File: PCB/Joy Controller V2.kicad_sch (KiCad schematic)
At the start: 36 parts, among them J1 Conn_02x16_Odd_Even, J4 USB_C_Receptacle_USB2.0_16P, SW1 SW_Push, SW10 SW_Push, SW11 SW_Push, SW12 SW_Push, SW13 SW_Push, SW2 SW_Push, SW3 SW_Push, SW4 SW_Push, SW5 SW_Push, SW6 SW_Push, SW7 SW_Push, SW8 SW_Push, SW9 SW_Push, U1 COM-09032, U2 COM-09032

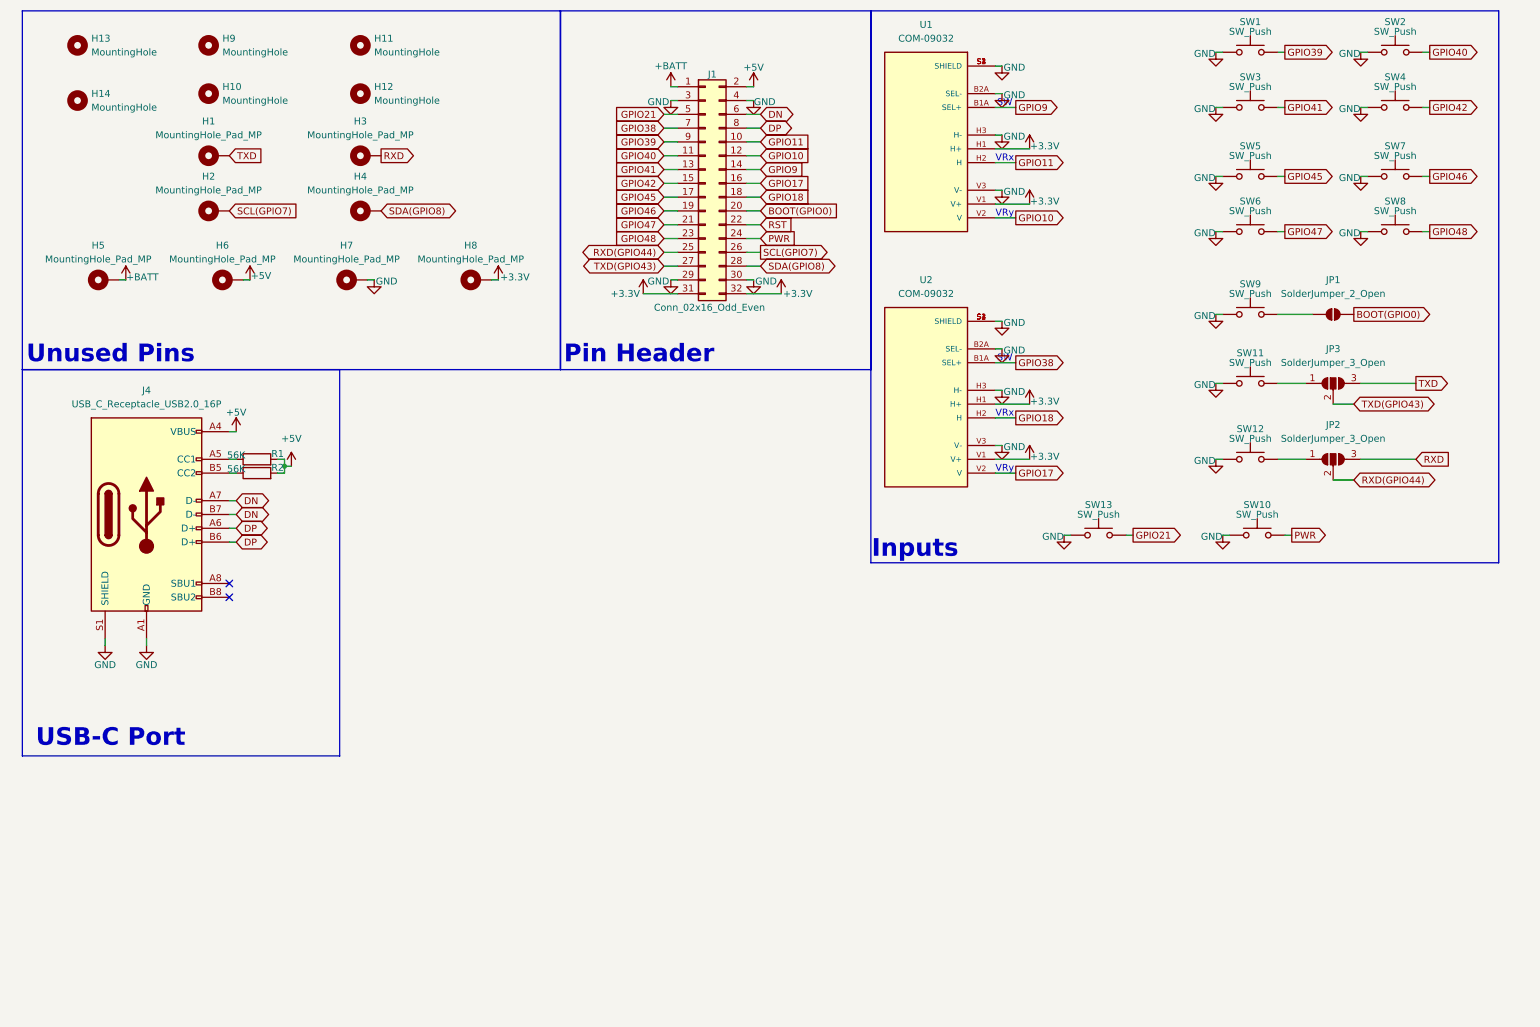
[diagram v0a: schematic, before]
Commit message: Add files via upload
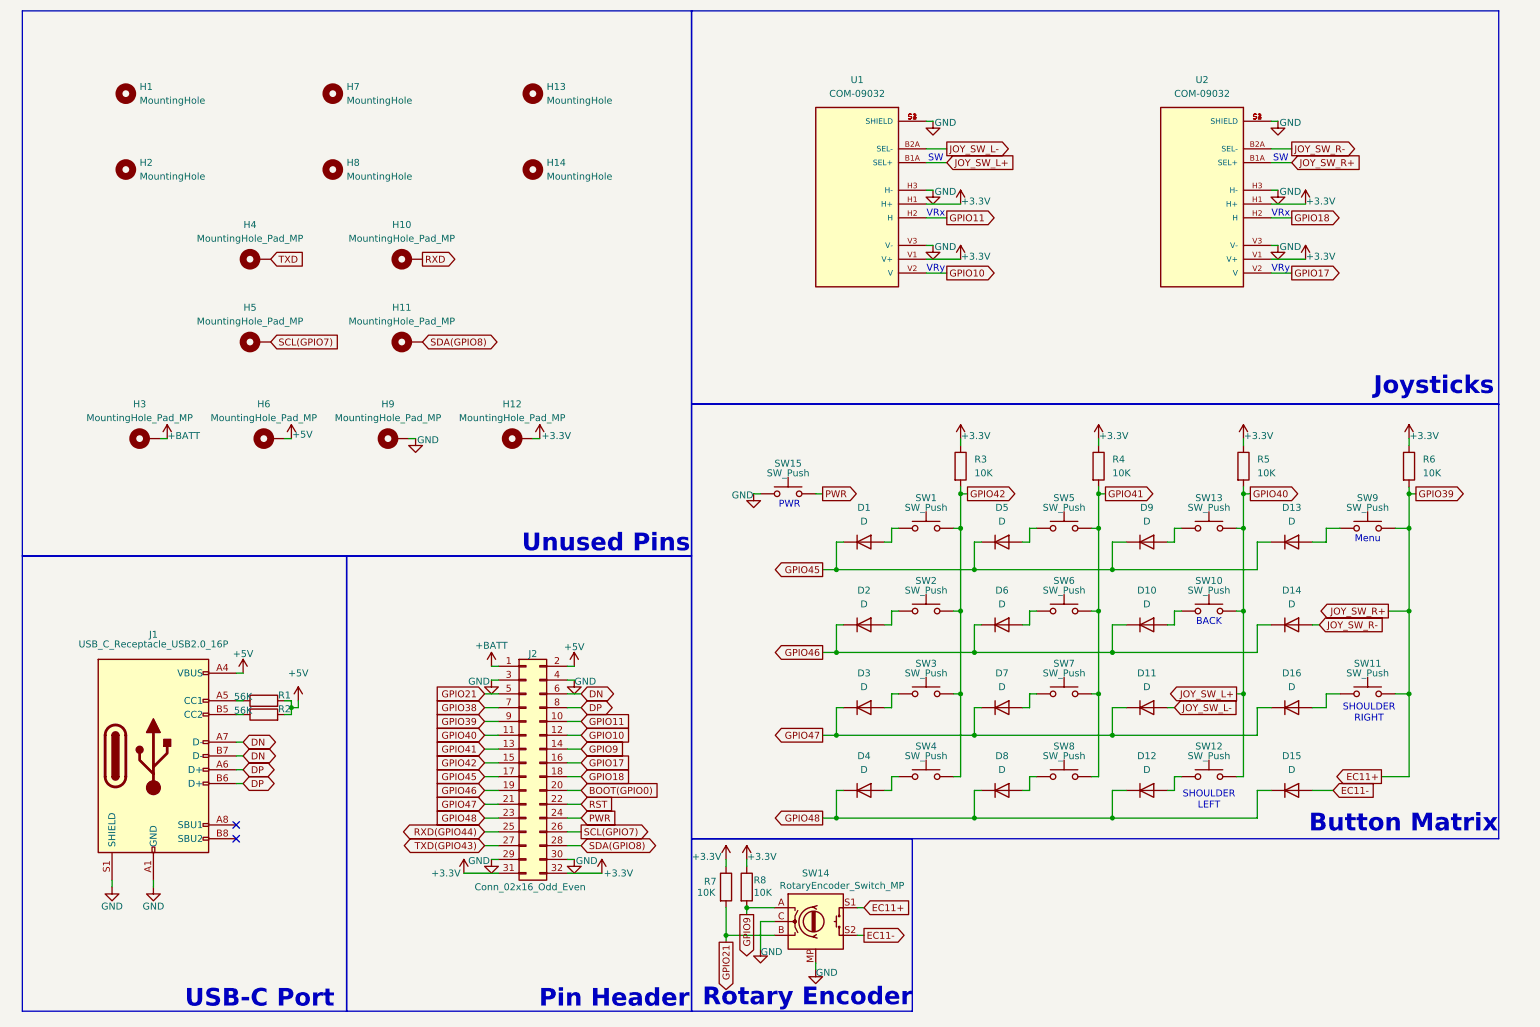
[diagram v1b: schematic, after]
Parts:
- removed JP1: SolderJumper_2_Open, Jumper:SolderJumper-2_P1.3mm_Open_RoundedPad1.0x1.5mm, symbol Jumper:SolderJumper_2_Open
- removed JP2, JP3: SolderJumper_3_Open, Jumper:SolderJumper-3_P1.3mm_Open_RoundedPad1.0x1.5mm, symbol Jumper:SolderJumper_3_Open
- added D1, D10, D11, D12, D13, D14, D15, D16, D2, D3, D4, D5, D6, D7, D8, D9: D, Diode_SMD:D_SOD-323, symbol Device:D
- added R3, R4, R5, R6, R7, R8: 10K, Resistor_SMD:R_0603_1608Metric, symbol Device:R
- added SW13: SW_Push, Button_Switch_THT:SW_Tactile_SKHH_Angled, symbol Switch:SW_Push
- added SW14: RotaryEncoder_Switch_MP, Rotary_Encoder:RotaryEncoder_Alps_EC11E-Switch_Vertical_H20mm, symbol Device:RotaryEncoder_Switch_MP
- renumbered H13 to H1, H3 to H10, H4 to H11, H8 to H12, H11 to H13, H12 to H14, H14 to H2, H5 to H3, H1 to H4, H2 to H5, H9 to H7, H10 to H8, H7 to H9, J4 to J1, J1 to J2, SW9 to SW10, SW10 to SW15, SW3 to SW2, SW5 to SW3, SW7 to SW4, SW2 to SW5, SW4 to SW6, SW6 to SW7, SW13 to SW9
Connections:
- net +3.3V: now also R3.1, R4.1, R5.1, R6.1, R7.1, R8.1
- net GND: now also SW14.C, SW14.MP; no longer SW1.1, SW10.1, SW11.1, SW12.1, SW2.1, SW3.1, SW4.1, SW5.1, SW6.1, SW7.1, SW8.1, SW9.1, U1.B2A (SEL-), U2.B2A (SEL-)
- net GPIO21: now also R7.2, SW14.B; no longer SW9.2
- net GPIO38: no longer U2.B1A (SEL+)
- net GPIO40: now also SW10.2, SW12.2, U1.B1A (SEL+), R5.2, SW13.2; no longer SW5.2
- net GPIO41: now also SW5.2, SW6.2, SW7.2, SW8.2, R4.2; no longer SW2.2
- net GPIO42: now also SW1.2, SW2.2, SW3.2, SW4.2, R3.2; no longer SW6.2
- net GPIO45: now also D1.1 (K), D13.1 (K), D5.1 (K), D9.1 (K); no longer SW3.2
- net GPIO46: now also D10.1 (K), D14.1 (K), D2.1 (K), D6.1 (K); no longer SW4.2
- net GPIO47: now also D11.1 (K), D16.1 (K), D3.1 (K), D7.1 (K); no longer SW7.2
- net GPIO48: now also D12.1 (K), D15.1 (K), D4.1 (K), D8.1 (K); no longer SW8.2
- net GPIO9: now also R8.2, SW14.A; no longer U1.B1A (SEL+)
- net EC11+: now reaches SW11.2
- net EC11+: now also J2.9 (Pin_9), SW9.2, U2.B1A (SEL+), R6.2, SW14.S1
- removed net GPIO39: J2.9 (Pin_9), SW1.2
- new net: D13.2 (A), SW9.1
- new net: D16.2 (A), SW11.1
- new net: D9.2 (A), SW13.1
- new net: D4.2 (A), SW4.1
- new net: D7.2 (A), SW7.1
- new net: D1.2 (A), SW1.1
- new net: D6.2 (A), SW6.1
- new net: D8.2 (A), SW8.1
- new net: D10.2 (A), SW10.1
- new net: D12.2 (A), SW12.1
- new net: D3.2 (A), SW3.1
- new net: D2.2 (A), SW2.1
- new net: D5.2 (A), SW5.1
- new net EC11-: D15.2 (A), SW14.S2
- new net JOY_SW_L-: D11.2 (A), U1.B2A (SEL-)
- new net JOY_SW_R-: D14.2 (A), U2.B2A (SEL-)
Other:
- note added: "BACK"
- note added: "Button Matrix"
- note added: "Joysticks"
- note added: "Menu"
- note added: "PWR"
- note added: "Rotary Encoder"
- note added: "SHOULDER LEFT"
- note added: "SHOULDER RIGHT"
- note removed: "Inputs"
- moved on the sheet: H1, H10, H11, H12, H13, H14, H2, H3, H4, H5, H6, H7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

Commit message: Add files via upload
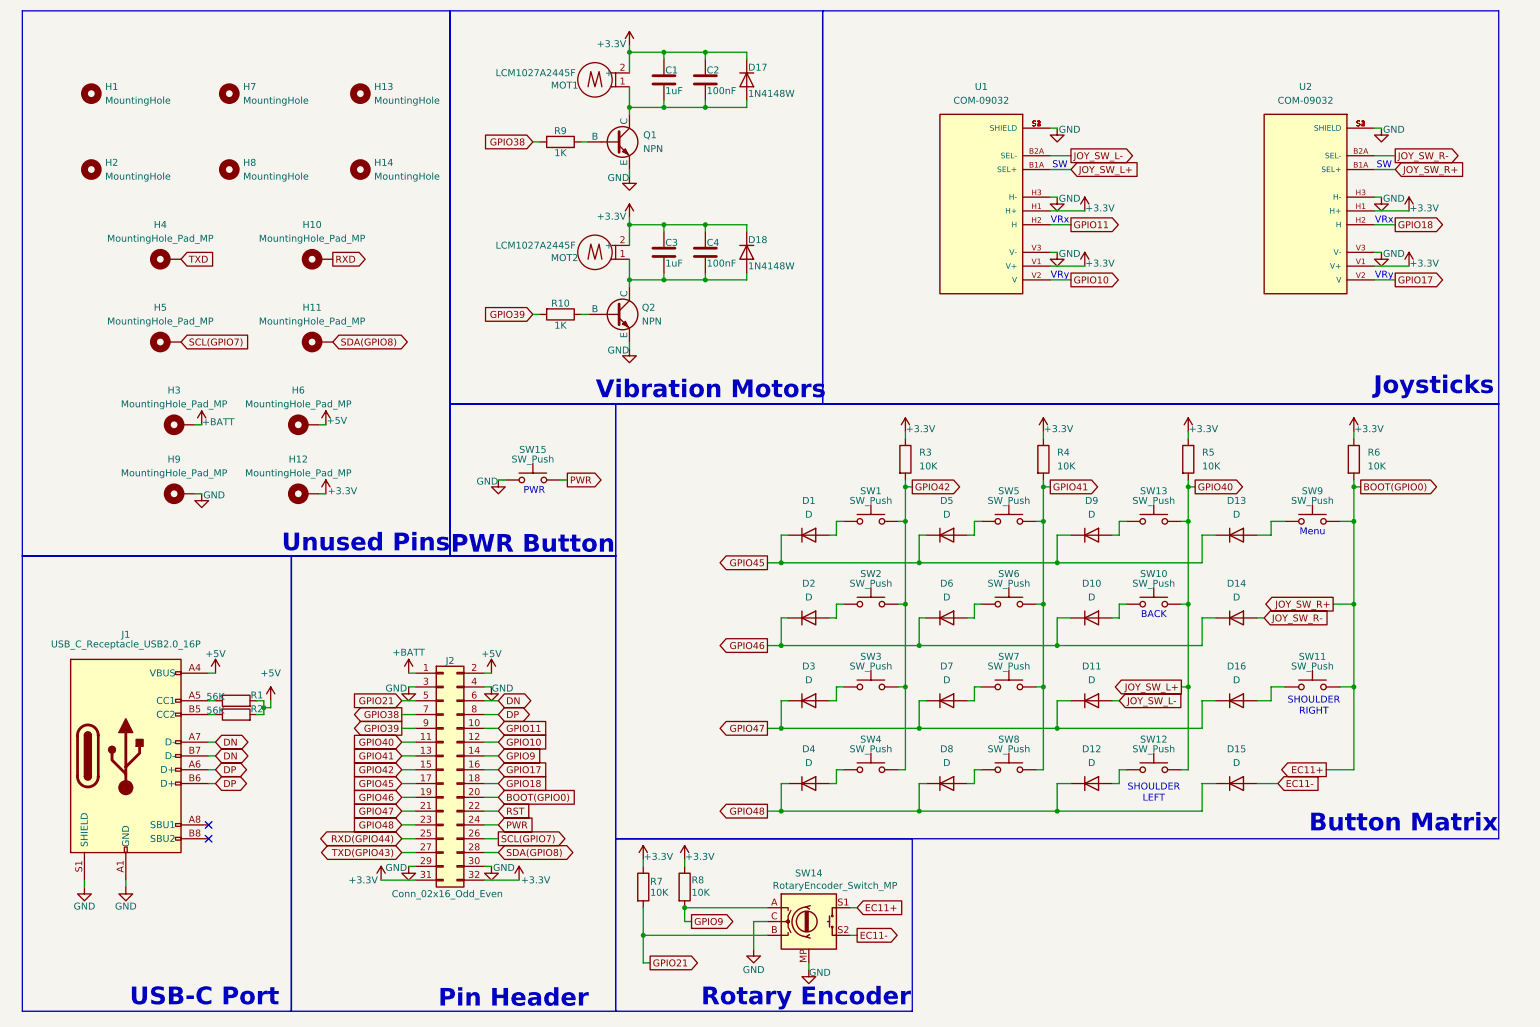
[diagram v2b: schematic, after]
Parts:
- added C1, C3: 1uF, Capacitor_SMD:C_0603_1608Metric, symbol Device:C
- added C2, C4: 100nF, Capacitor_SMD:C_0603_1608Metric, symbol Device:C
- added D17, D18: 1N4148W, Diode_SMD:D_SOD-123, symbol Diode:1N4148W
- added MOT1, MOT2: LCM1027A2445F, lcsc:VIBRATING-MOTOR-SMD_WELDING, symbol lcsc:LCM1027A2445F
- added Q1, Q2: NPN, Package_TO_SOT_SMD:SOT-23, symbol Simulation_SPICE:NPN
- added R10, R9: 1K, Resistor_SMD:R_0603_1608Metric, symbol Device:R
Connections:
- net +3.3V: now also C1.2, C2.2, C3.2, C4.2, D17.1 (K), D18.1 (K), MOT1.2 (+), MOT2.2 (+)
- net BOOT(GPIO0): now also R6.2, SW11.2, SW14.S1, SW9.2, U2.B1A (SEL+)
- net GND: now also Q1.3 (E), Q2.3 (E)
- net GPIO38: now also R9.2
- removed net EC11+: J2.9 (Pin_9), R6.2, SW11.2, SW14.S1, SW9.2, U2.B1A (SEL+)
- new net: C1.1, C2.1, D17.2 (A), MOT1.1 (-), Q1.1 (C)
- new net: Q1.2 (B), R9.1
- new net: Q2.2 (B), R10.1
- new net: C3.1, C4.1, D18.2 (A), MOT2.1 (-), Q2.1 (C)
- new net GPIO39: J2.9 (Pin_9), R10.2
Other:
- note added: "PWR Button"
- note added: "Vibration Motors"
- moved on the sheet: D1, D10, D11, D12, D13, D14, D15, D16, D2, D3, D4, D5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

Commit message: Add files via upload
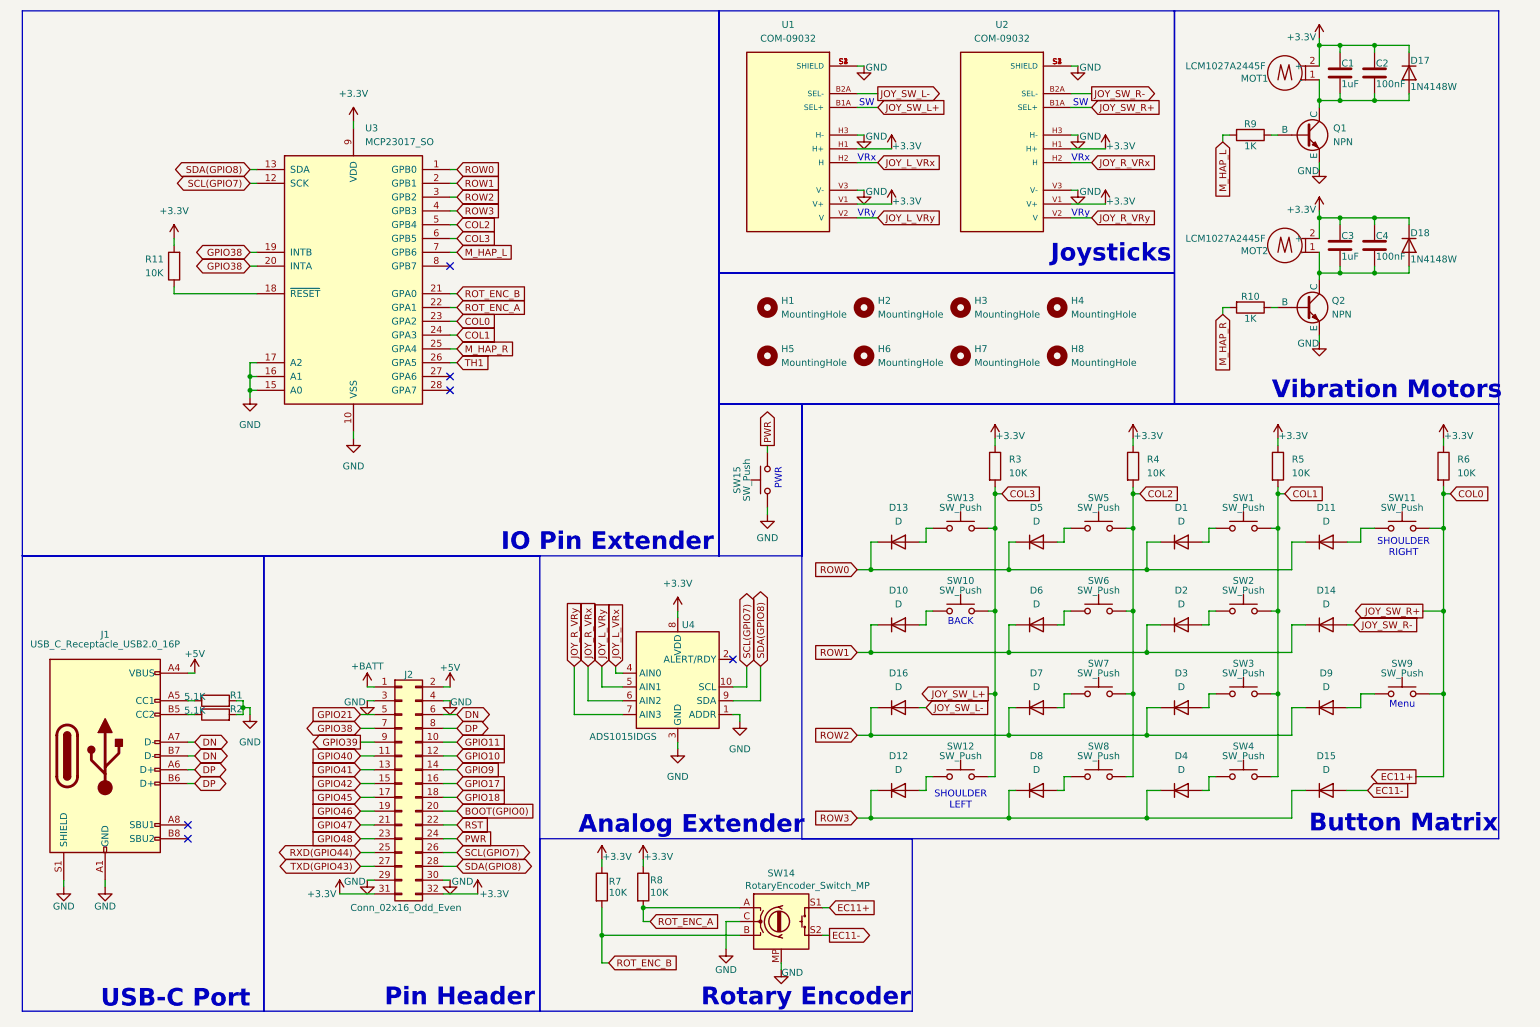
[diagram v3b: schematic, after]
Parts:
- removed H10, H11, H12, H3, H4, H5, H6, H9: MountingHole_Pad_MP, symbol Mechanical:MountingHole_Pad_MP
- added H5, H6: MountingHole, MountingHole:MountingHole_2mm, symbol Mechanical:MountingHole
- added R11: 10K, Resistor_SMD:R_0603_1608Metric, symbol Device:R
- added U3: MCP23017_SO, Package_SO:SOIC-28W_7.5x17.9mm_P1.27mm, symbol Interface_Expansion:MCP23017_SO
- added U4: ADS1015IDGS, Package_SO:TSSOP-10_3x3mm_P0.5mm, symbol Analog_ADC:ADS1015IDGS
- R1, R2: value 56K -> 5.1K
- renumbered D9 to D1, D2 to D10, D13 to D11, D4 to D12, D1 to D13, D3 to D16, D10 to D2, D11 to D3, D12 to D4, D16 to D9, H8 to H1, H13 to H2, H2 to H3, H7 to H4, H1 to H7, H14 to H8
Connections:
- net +3.3V: now also R11.2, U3.9 (VDD), U4.8 (VDD)
- net +5V: no longer R1.2, R2.2
- net BOOT(GPIO0): no longer R6.2, SW11.2, SW14.S1, SW9.2, U2.B1A (SEL+)
- net GND: now also R1.2, R2.2, U3.10 (VSS), U3.15 (A0), U3.16 (A1), U3.17 (A2), U4.1 (ADDR), U4.3 (GND)
- net GPIO10: no longer U1.V2 (V)
- net GPIO11: no longer U1.H2 (H)
- net GPIO17: no longer U2.V2 (V)
- net GPIO18: no longer U2.H2 (H)
- net GPIO21: no longer R7.2, SW14.B
- net GPIO38: now also U3.19 (INTB), U3.20 (INTA); no longer R9.2
- net GPIO39: no longer R10.2
- net GPIO40: no longer R5.2, SW10.2, SW12.2, SW13.2, U1.B1A (SEL+)
- net GPIO41: no longer R4.2, SW5.2, SW6.2, SW7.2, SW8.2
- net GPIO42: no longer R3.2, SW1.2, SW2.2, SW3.2, SW4.2
- net GPIO45: no longer D1.1 (K), D11.1 (K), D13.1 (K), D5.1 (K)
- net GPIO46: no longer D10.1 (K), D14.1 (K), D2.1 (K), D6.1 (K)
- net GPIO47: no longer D16.1 (K), D3.1 (K), D7.1 (K), D9.1 (K)
- net GPIO48: no longer D12.1 (K), D15.1 (K), D4.1 (K), D8.1 (K)
- net GPIO9: no longer R8.2, SW14.A
- net JOY_SW_L-: now also D16.2 (A); no longer D3.2 (A)
- net SCL(GPIO7): now also U3.12 (SCK), U4.10 (SCL)
- net SDA(GPIO8): now also U3.13 (SDA), U4.9 (SDA)
- net at SW9.1: now also D9.2 (A); no longer D11.2 (A)
- net at SW11.1: now also D11.2 (A); no longer D9.2 (A)
- net at SW13.1: now also D13.2 (A); no longer D1.2 (A)
- net at SW4.1: now also D4.2 (A); no longer D12.2 (A)
- net at SW1.1: now also D1.2 (A); no longer D13.2 (A)
- net at D2.2 (A): now also SW2.1; no longer SW10.1
- net at SW12.1: now also D12.2 (A); no longer D4.2 (A)
- net at SW3.1: now also D3.2 (A); no longer D16.2 (A)
- net at D10.2 (A): now also SW10.1; no longer SW2.1
- new net: R11.1, U3.18 (~{RESET})
- new net COL0: R6.2, SW11.2, SW14.S1, SW9.2, U2.B1A (SEL+), U3.23 (GPA2)
- new net COL1: R5.2, SW1.2, SW2.2, SW3.2, SW4.2, U3.24 (GPA3)
- new net COL2: R4.2, SW5.2, SW6.2, SW7.2, SW8.2, U3.5 (GPB4)
- new net COL3: R3.2, SW10.2, SW12.2, SW13.2, U1.B1A (SEL+), U3.6 (GPB5)
- new net JOY_L_VRx: U1.H2 (H), U4.4 (AIN0)
- new net JOY_L_VRy: U1.V2 (V), U4.5 (AIN1)
- new net JOY_R_VRx: U2.H2 (H), U4.6 (AIN2)
- new net JOY_R_VRy: U2.V2 (V), U4.7 (AIN3)
- new net M_HAP_L: R9.2, U3.7 (GPB6)
- new net M_HAP_R: R10.2, U3.25 (GPA4)
- new net ROT_ENC_A: R8.2, SW14.A, U3.22 (GPA1)
- new net ROT_ENC_B: R7.2, SW14.B, U3.21 (GPA0)
- new net ROW0: D1.1 (K), D11.1 (K), D13.1 (K), D5.1 (K), U3.1 (GPB0)
- new net ROW1: D10.1 (K), D14.1 (K), D2.1 (K), D6.1 (K), U3.2 (GPB1)
- new net ROW2: D16.1 (K), D3.1 (K), D7.1 (K), D9.1 (K), U3.3 (GPB2)
- new net ROW3: D12.1 (K), D15.1 (K), D4.1 (K), D8.1 (K), U3.4 (GPB3)
- new net TH1: U3.26 (GPA5)
- no-connect marks 2 -> 6
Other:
- note added: "Analog Extender"
- note added: "IO Pin Extender"
- note removed: "PWR Button"
- note removed: "Unused Pins"
- moved on the sheet: C1, C2, C3, C4, D1, D10, D11, D12, D13, D14, D15, D16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
